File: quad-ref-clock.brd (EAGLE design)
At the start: 46 x 48.5 mm, 29 parts, among them U1 LMK00804B, U2 ADP150, U3 ADP150, X1 SMA, X2 SMA, X3 SMA, X4 SMA

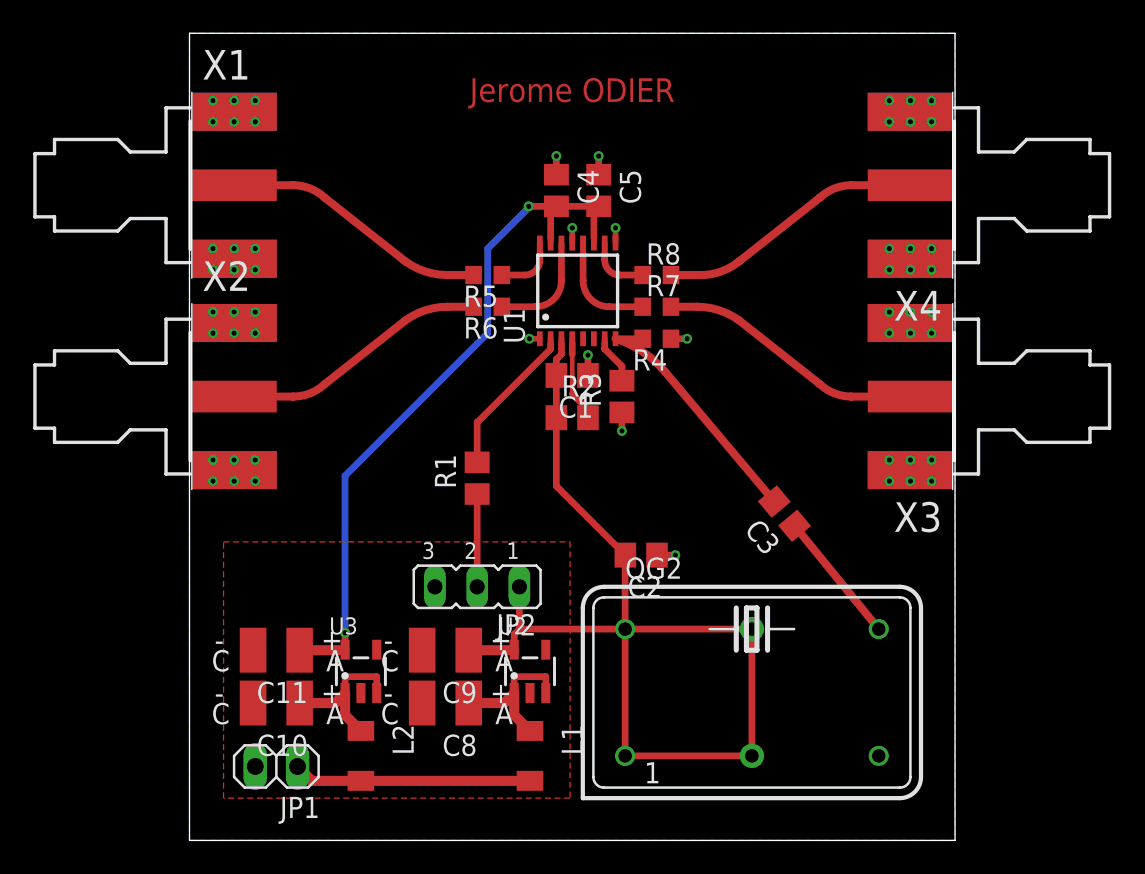
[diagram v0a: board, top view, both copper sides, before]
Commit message: update
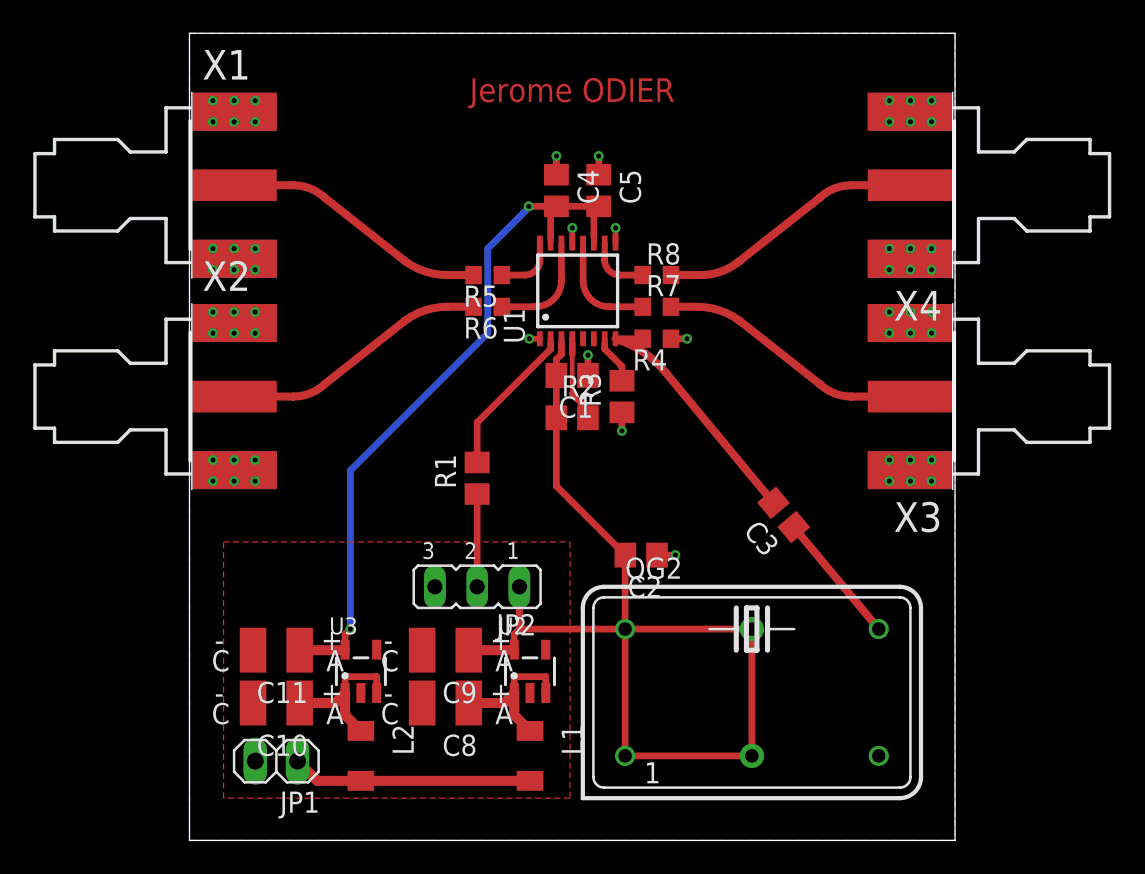
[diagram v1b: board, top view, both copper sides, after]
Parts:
- moved JP1 0.32 mm to (5.08, 4.76)
- moved C3 0.09 mm to (35.6, 19.6)
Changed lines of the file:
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@@
 <setting verticaltext="up"/>
 </settings>
-<grid distance="0.0125" unitdist="inch" unit="inch" style="lines" multiple="1" display="yes" altdistance="0.025" altunitdist="inch" altunit="inch"/>
+<grid distance="0.025" unitdist="inch" unit="inch" style="lines" multiple="1" display="yes" altdistance="0.025" altunitdist="inch" altunit="inch"/>
 <layers>
 <layer number="1" name="Top" color="4" fill="1" visible="yes" active="yes"/>
@@
 <element name="C11" library="radiotelescope" package="CAPACITOR_POL_1210" value="1u" x="5.08" y="11.43" rot="R180"/>
 <element name="C2" library="rcl" package="C0805" value="100n" x="27.0002" y="17.145" rot="R180"/>
-<element name="C3" library="rcl" package="C0805" value="470pF" x="35.6108" y="19.6342" rot="R130"/>
+<element name="C3" library="rcl" package="C0805" value="470pF" x="35.56" y="19.558" rot="R130"/>
 <element name="C4" library="rcl" package="C0805" value="100n" x="21.9075" y="39.0525" rot="R270"/>
 <element name="C5" library="rcl" package="C0805" value="100n" x="24.4475" y="39.0525" rot="R270"/>
 <element name="C8" library="radiotelescope" package="CAPACITOR_POL_1210" value="1u" x="15.24" y="8.255" rot="R180"/>
 <element name="C9" library="radiotelescope" package="CAPACITOR_POL_1210" value="1u" x="15.24" y="11.43" rot="R180"/>
-<element name="JP1" library="pinhead" package="1X02" value="" x="5.08" y="4.445" rot="R180"/>
+<element name="JP1" library="pinhead" package="1X02" value="" x="5.08" y="4.7625" rot="R180"/>
 <element name="JP2" library="jumper" package="JP2" value="" x="17.145" y="15.24" rot="R180"/>
 <element name="L1" library="rcl" package="L3216C" value="MI1206K601R−10" x="20.32" y="5.08" rot="R270"/>
@@
 <wire x1="9.1799" y1="11.43" x2="9.21" y2="11.4601" width="0.4064" layer="1"/>
 <wire x1="9.21" y1="11.4601" x2="9.2075" y2="11.4601" width="0.4064" layer="1"/>
-<wire x1="9.2075" y1="11.4601" x2="9.2075" y2="12.4714" width="0.4064" layer="1"/>
-<via x="9.2075" y="12.4714" extent="1-16" drill="0.3048"/>
+<via x="9.525" y="12.7" extent="1-16" drill="0.3048"/>
 <contactref element="C4" pad="2"/>
 <contactref element="C5" pad="2"/>
@@
 <wire x1="17.78" y1="35.56" x2="20.32" y2="38.1" width="0.4064" layer="16"/>
 <wire x1="20.32" y1="38.1" x2="20.2438" y2="38.1" width="0.4064" layer="16"/>
-<wire x1="9.2075" y1="12.4714" x2="9.2075" y2="21.9075" width="0.4064" layer="16"/>
-<wire x1="9.2075" y1="21.9075" x2="17.78" y2="30.48" width="0.4064" layer="16"/>
+<wire x1="9.525" y1="22.225" x2="17.78" y2="30.48" width="0.4064" layer="16"/>
+<wire x1="9.2075" y1="11.4601" x2="9.2075" y2="12.3825" width="0.4064" layer="1"/>
+<wire x1="9.2075" y1="12.3825" x2="9.525" y2="12.7" width="0.4064" layer="1"/>
+<wire x1="9.525" y1="12.7" x2="9.525" y2="22.225" width="0.4064" layer="16"/>
 </signal>
 <signal name="N$7">
 <contactref element="U1" pad="8"/>
 <contactref element="C3" pad="2"/>
-<wire x1="35.00015" y1="20.361940625" x2="28.4734" y2="28.1178" width="0.4826" layer="1"/>
+<wire x1="34.94935" y1="20.285740625" x2="28.4734" y2="28.1178" width="0.4826" layer="1"/>
 <contactref element="R4" pad="2"/>
 <wire x1="28.4734" y1="28.1178" x2="25.46" y2="30.145" width="0.4826" layer="1" curve="32.978915" cap="flat"/>
@@
 <contactref element="C3" pad="1"/>
 <contactref element="QG2" pad="8"/>
-<wire x1="41.275" y1="12.7" x2="36.221446875" y2="18.90645625" width="0.4826" layer="1"/>
+<wire x1="41.275" y1="12.7" x2="36.170646875" y2="18.83025625" width="0.4826" layer="1"/>
 </signal>
 <signal name="N$16">
@@
 <contactref element="JP1" pad="1"/>
 <wire x1="10.16" y1="3.58" x2="20.32" y2="3.58" width="0.6096" layer="1"/>
-<wire x1="10.16" y1="3.58" x2="7.215" y2="3.58" width="0.6096" layer="1"/>
-<wire x1="7.215" y1="3.58" x2="6.35" y2="4.445" width="0.6096" layer="1"/>
+<wire x1="10.16" y1="3.58" x2="7.5325" y2="3.58" width="0.6096" layer="1"/>
+<wire x1="7.5325" y1="3.58" x2="6.35" y2="4.7625" width="0.6096" layer="1"/>
 </signal>
 <signal name="N$14">
